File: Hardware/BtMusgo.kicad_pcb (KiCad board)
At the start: 2 copper layers, 123 x 82.7 mm, 36 parts, among them IC1 ArduinoProMini, J1 Power, J2 microSD, J3 RTC, J4 SHT71, Q1 2N3904, Q2 2N3904, U1 TLC274, U2 TLC274, U3 LM1117-3.3

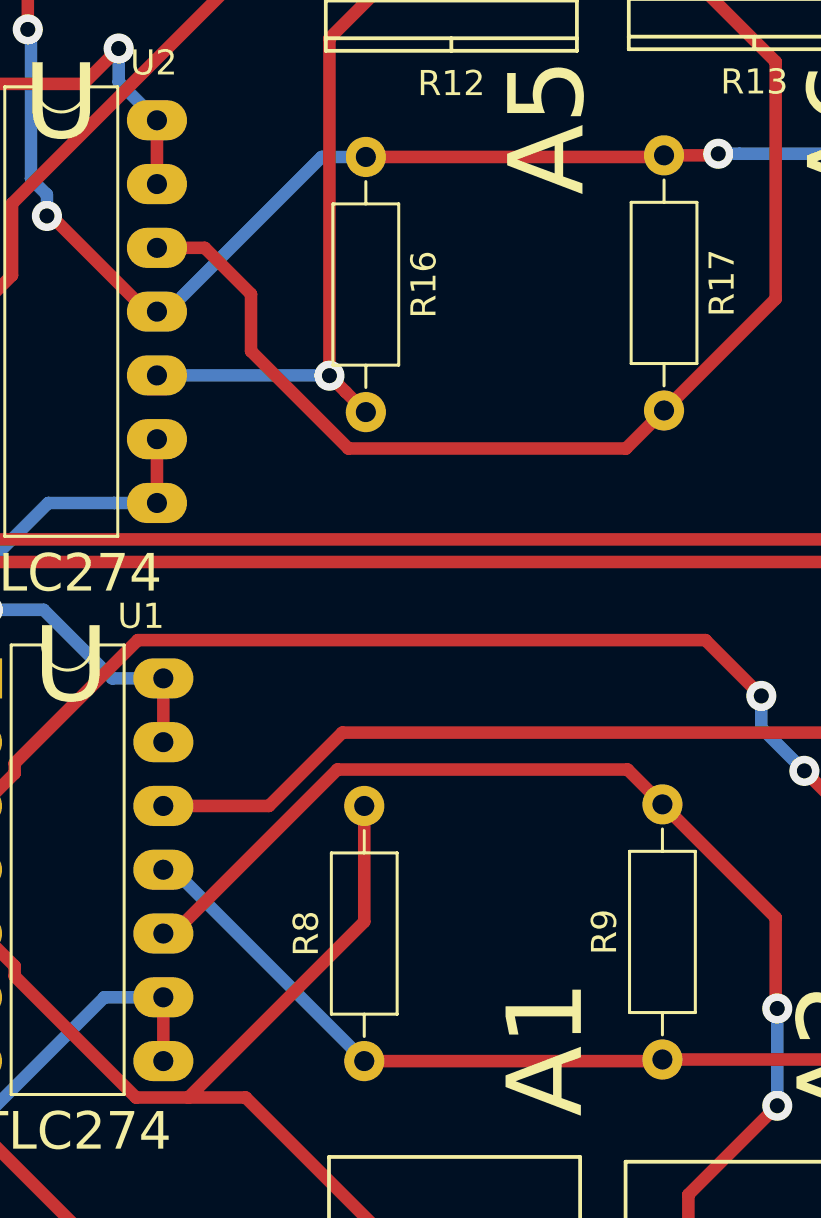
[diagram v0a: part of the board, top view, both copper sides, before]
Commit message: Bug fixes
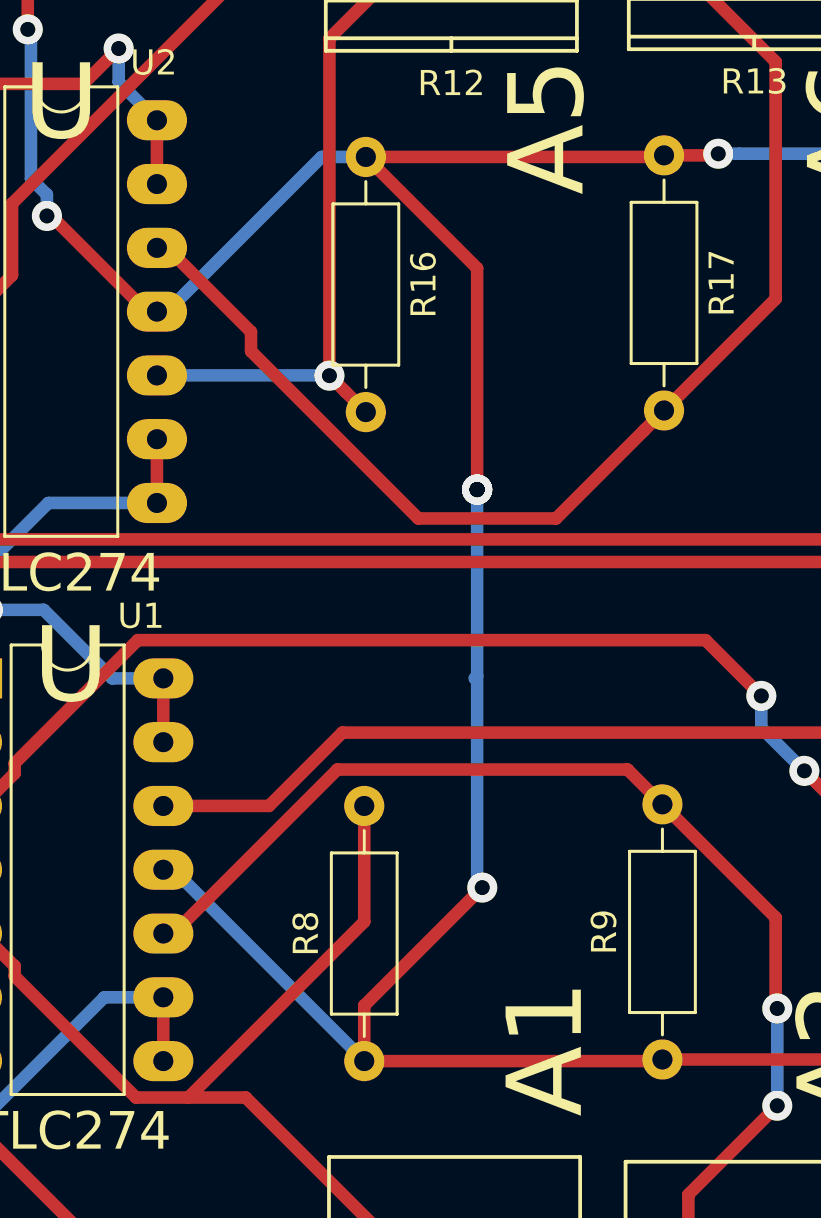
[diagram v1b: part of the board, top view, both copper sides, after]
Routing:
- net ON_GND: track 143.6 -> 183.6 mm, vias 7 -> 11
- net Net-(R13-Pad1): track 47.7 -> 49.1 mm
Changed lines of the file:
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@@
-(kicad_pcb (version 4) (host pcbnew 4.0.7-e2-6376~58~ubuntu14.04.1)
+(kicad_pcb (version 4) (host pcbnew 4.0.2+dfsg1-stable)
   (general
     (links 85)
     (no_connects 1)
-    (area 123.165799 69.165399 246.302601 151.967001)
+    (area 115.9256 64.8716 252.425858 154.025601)
     (thickness 1.6)
     (drawings 75)
-    (tracks 502)
+    (tracks 514)
     (zones 0)
     (modules 36)
@@
   (segment (start 158.75 73.914) (end 163.703 73.914) (width 0.5) (layer F.Cu) (net 31))
   (segment (start 163.703 73.914) (end 164.465 73.152) (width 0.5) (layer F.Cu) (net 31))
+  (segment (start 205.994 118.5672) (end 201.295 123.2662) (width 0.5) (layer F.Cu) (net 32))
+  (segment (start 201.295 123.2662) (end 201.295 125.476) (width 0.5) (layer F.Cu) (net 32))
+  (segment (start 205.7908 102.7176) (end 205.7908 118.364) (width 0.5) (layer B.Cu) (net 32))
+  (segment (start 205.7908 118.364) (end 205.994 118.5672) (width 0.5) (layer B.Cu) (net 32))
+  (via (at 205.994 118.5672) (size 1.2) (drill 0.6) (layers F.Cu B.Cu) (net 32))
+  (via (at 205.7908 102.7176) (size 1.2) (drill 0.6) (layers F.Cu B.Cu) (net 32))
+  (via (at 205.7908 102.7176) (size 1.2) (drill 0.6) (layers F.Cu B.Cu) (net 32))
+  (segment (start 205.7908 110.1344) (end 205.6892 110.236) (width 0.5) (layer B.Cu) (net 32))
+  (segment (start 201.3585 89.4715) (end 205.7908 93.9038) (width 0.5) (layer F.Cu) (net 32))
+  (via (at 205.7908 102.7176) (size 1.2) (drill 0.6) (layers F.Cu B.Cu) (net 32))
+  (segment (start 205.7908 93.9038) (end 205.7908 102.7176) (width 0.5) (layer F.Cu) (net 32))
   (segment (start 231.648 89.281) (end 237.1725 89.281) (width 0.5) (layer F.Cu) (net 32))
   (segment (start 237.1725 89.281) (end 237.236 89.3445) (width 0.5) (layer F.Cu) (net 32))
@@
   (segment (start 199.908499 98.181499) (end 200.558501 98.831501) (width 0.5) (layer F.Cu) (net 38))
   (segment (start 200.558501 98.831501) (end 201.3585 99.6315) (width 0.5) (layer F.Cu) (net 38))
+  (segment (start 208.933398 103.867602) (end 212.433001 100.367999) (width 0.5) (layer F.Cu) (net 39))
+  (segment (start 203.4486 103.867602) (end 208.933398 103.867602) (width 0.5) (layer F.Cu) (net 39))
+  (segment (start 196.7865 97.205502) (end 203.4486 103.867602) (width 0.5) (layer F.Cu) (net 39))
+  (segment (start 212.433001 100.367999) (end 213.233 99.568) (width 0.5) (layer F.Cu) (net 39))
+  (segment (start 193.44 93.091) (end 196.7865 96.4375) (width 0.5) (layer F.Cu) (net 39))
+  (segment (start 193.04 93.091) (end 193.44 93.091) (width 0.5) (layer F.Cu) (net 39))
+  (segment (start 196.7865 96.4375) (end 196.7865 97.205502) (width 0.5) (layer F.Cu) (net 39))
   (segment (start 217.678 95.123) (end 217.678 85.6805) (width 0.5) (layer F.Cu) (net 39))
   (segment (start 217.678 85.6805) (end 214.329 82.3315) (width 0.5) (layer F.Cu) (net 39))
   (segment (start 213.233 99.568) (end 217.678 95.123) (width 0.5) (layer F.Cu) (net 39))
   (segment (start 214.329 82.3315) (end 214.329 80.5815) (width 0.5) (layer F.Cu) (net 39))
-  (segment (start 193.04 93.091) (end 194.945 93.091) (width 0.5) (layer F.Cu) (net 39))
-  (segment (start 194.945 93.091) (end 196.7865 94.9325) (width 0.5) (layer F.Cu) (net 39))
-  (segment (start 196.7865 94.9325) (end 196.7865 97.205502) (width 0.5) (layer F.Cu) (net 39))
-  (segment (start 196.7865 97.205502) (end 200.662499 101.081501) (width 0.5) (layer F.Cu) (net 39))
-  (segment (start 200.662499 101.081501) (end 211.719499 101.081501) (width 0.5) (layer F.Cu) (net 39))
-  (segment (start 211.719499 101.081501) (end 213.233 99.568) (width 0.5) (layer F.Cu) (net 39))
   (segment (start 237.236 99.5045) (end 238.586001 98.154499) (width 0.5) (layer F.Cu) (net 40))
   (segment (start 238.586001 98.154499) (end 238.586001 82.602001) (width 0.5) (layer F.Cu) (net 40))

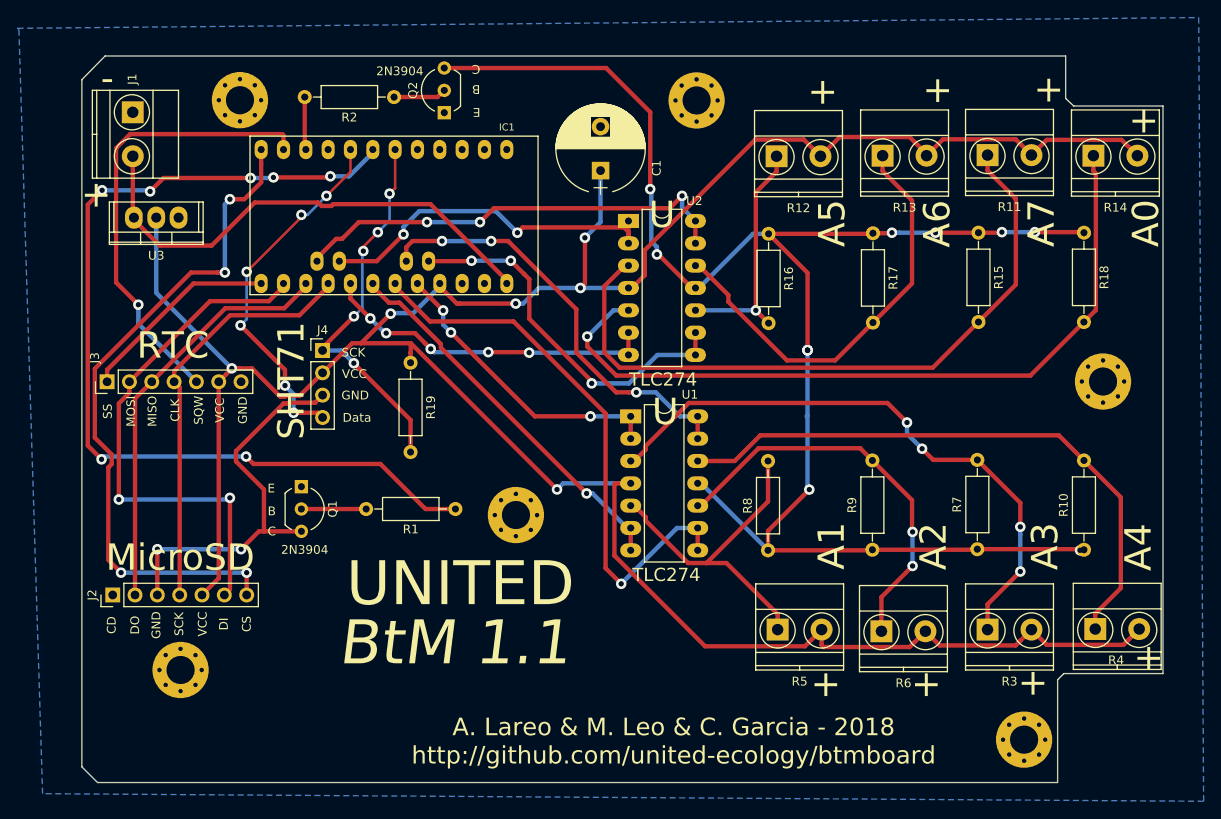
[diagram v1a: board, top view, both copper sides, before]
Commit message: Updates to v1.2
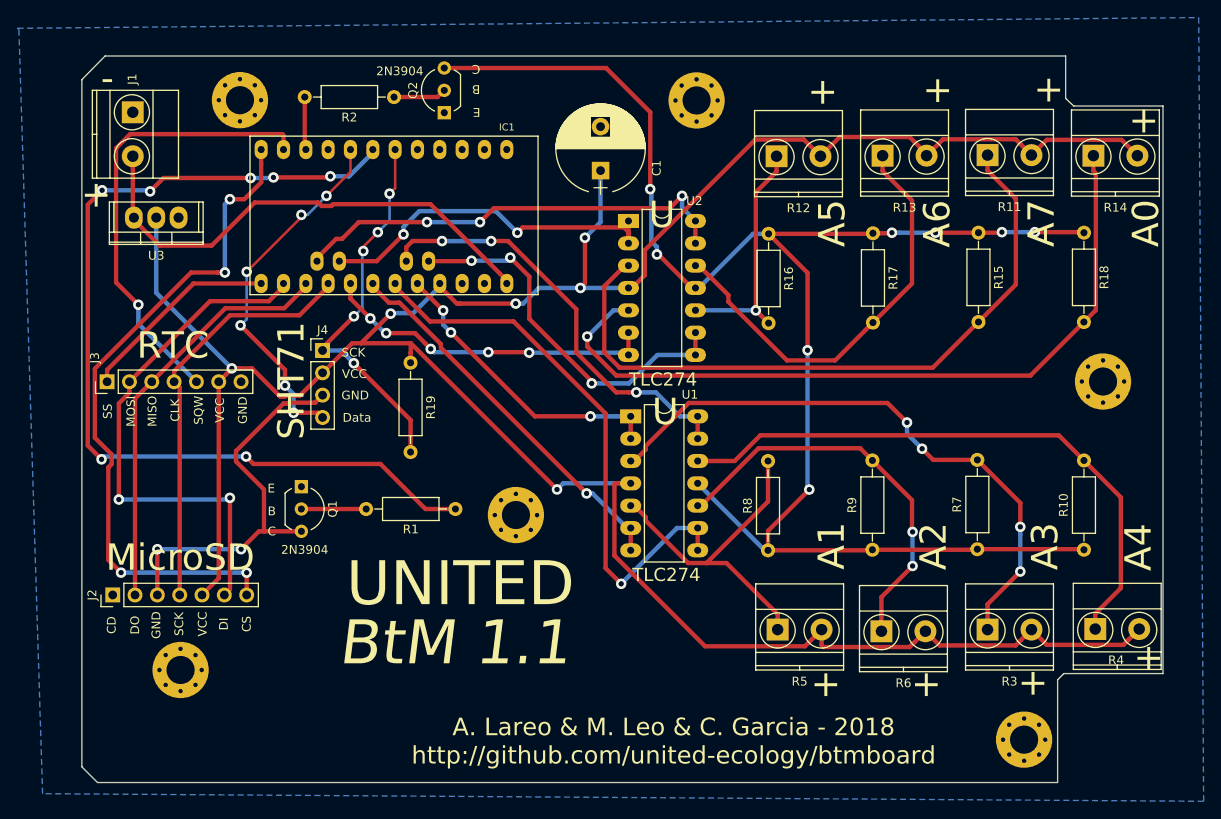
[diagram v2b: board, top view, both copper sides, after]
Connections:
- IC1 pad 1: Net-(IC1-Pad1) -> unconnected-(IC1-Pad1)
- IC1 pad 2: Net-(IC1-Pad2) -> unconnected-(IC1-Pad2)
- IC1 pad 22: Net-(IC1-Pad22) -> unconnected-(IC1-Pad22)
- IC1 pad 3: Net-(IC1-Pad3) -> unconnected-(IC1-Pad3)
- IC1 pad 5: Net-(IC1-Pad5) -> unconnected-(IC1-Pad5)
- IC1 pad 9: Net-(IC1-Pad9) -> unconnected-(IC1-Pad9)
- J2 pad 1: Net-(J2-Pad1) -> unconnected-(J2-Pad1)
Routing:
- net ON_GND: track 183.6 -> 181.4 mm, vias 11 -> 8
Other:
- net class Default removed
- rule pad_to_mask_clearance: 0.2 -> 0
